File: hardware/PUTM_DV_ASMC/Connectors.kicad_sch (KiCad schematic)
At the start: 7 parts, among them J1 FTSH-107-01-L-D-K, J2 IPBS-110-01-T-D-GP

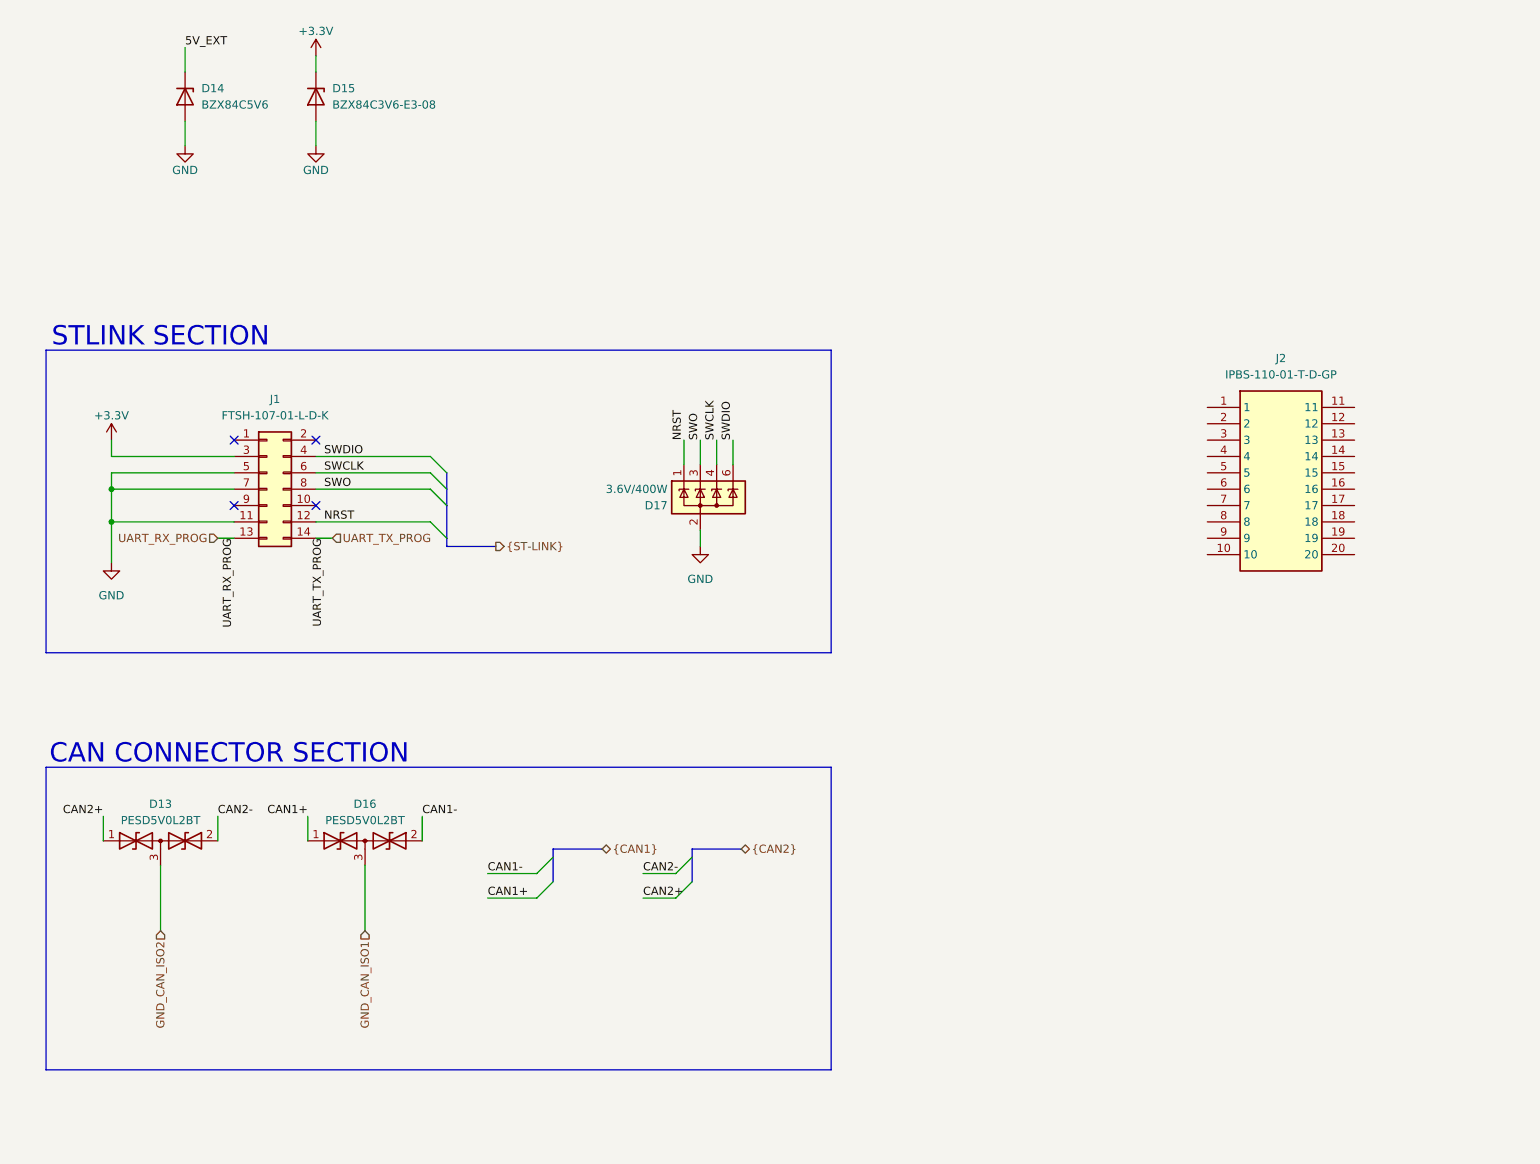
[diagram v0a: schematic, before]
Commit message: done schematic v1
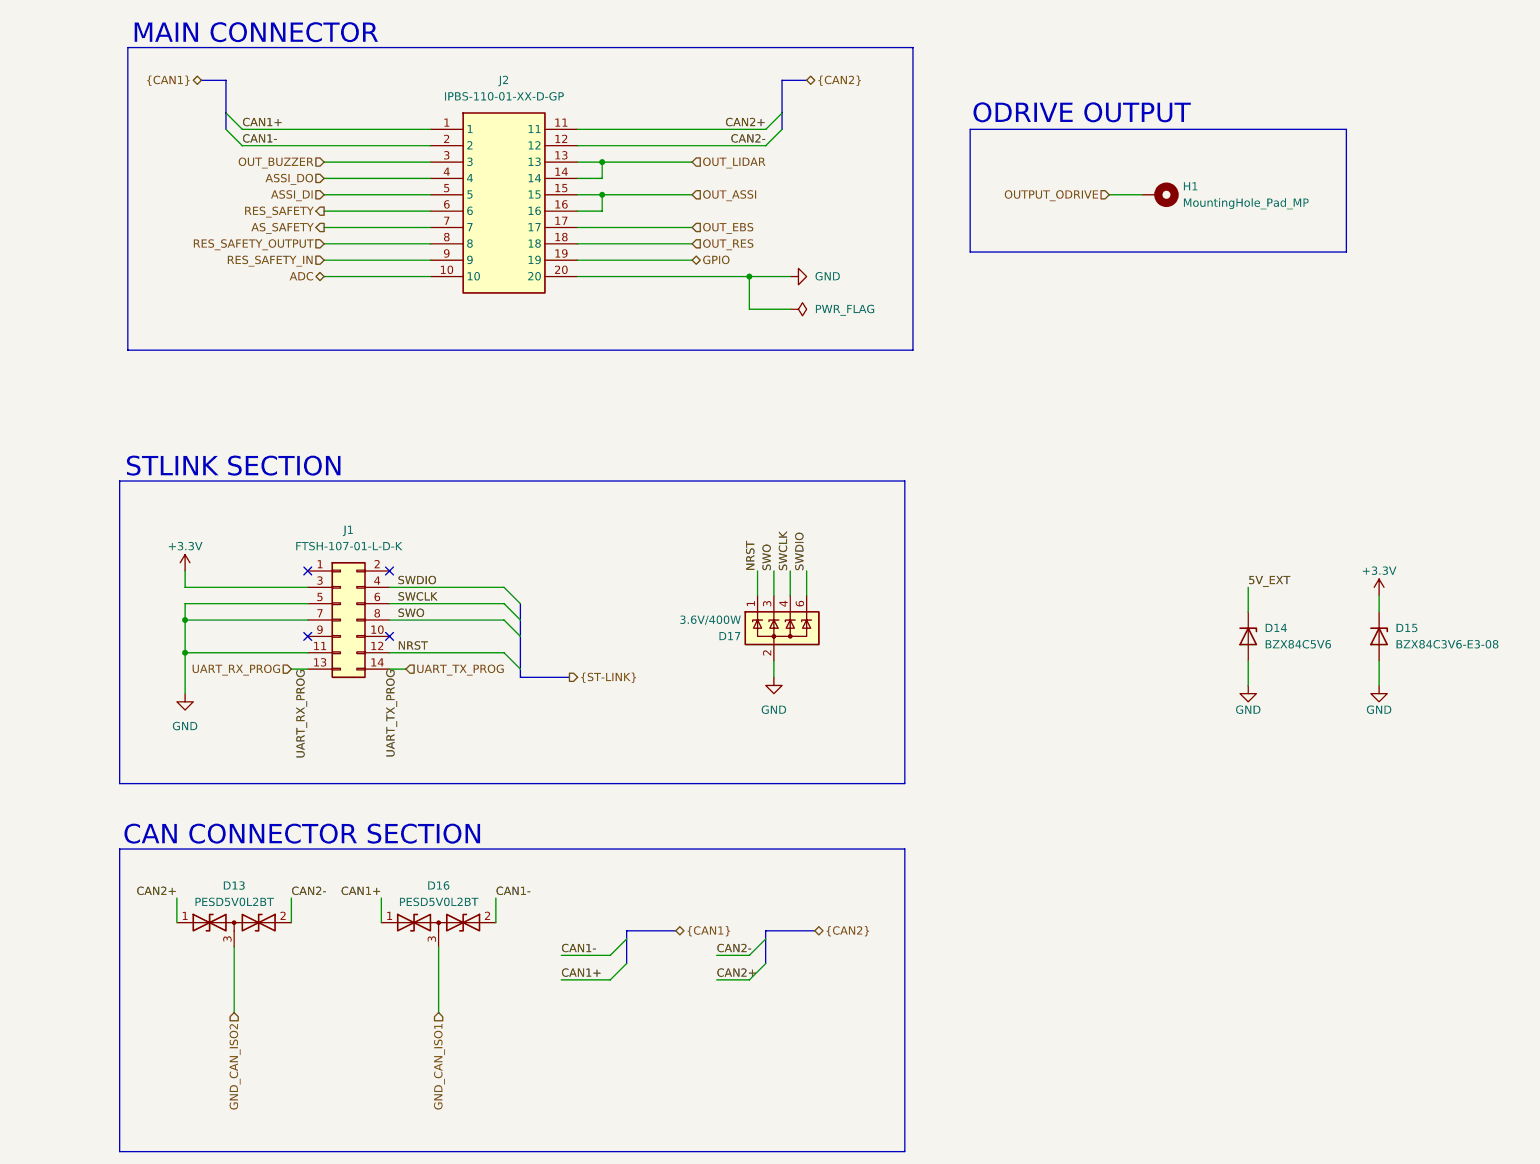
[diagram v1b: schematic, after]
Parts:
- removed J2: IPBS-110-01-T-D-GP, IPBS11001TDGP, symbol IPBS-110-01-T-D-GP:IPBS-110-01-T-D-GP
- added H1: MountingHole_Pad_MP, MountingHole:MountingHole_4.3mm_M4_DIN965_Pad_TopOnly, symbol Mechanical:MountingHole_Pad_MP
- added J2: IPBS-110-01-XX-D-GP, PDM:IPBT110H1TDRAGP, symbol PDM:IPBS-110-01-T-D-GP
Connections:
- net CAN1+: now also J2.1
- net CAN1-: now also J2.2
- net CAN2+: now also J2.11
- net CAN2-: now also J2.12
- net GND: now also J2.20
- new net ADC: J2.10
- new net ASSI_DI: J2.5
- new net ASSI_DO: J2.4
- new net AS_SAFETY: J2.7
- new net GPIO: J2.19
- new net OUTPUT_ODRIVE: H1.MP
- new net OUT_ASSI: J2.15, J2.16
- new net OUT_BUZZER: J2.3
- new net OUT_EBS: J2.17
- new net OUT_LIDAR: J2.13, J2.14
- new net OUT_RES: J2.18
- new net RES_SAFETY: J2.6
- new net RES_SAFETY_IN: J2.9
- new net RES_SAFETY_OUTPUT: J2.8
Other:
- note added: "MAIN CONNECTOR"
- note added: "ODRIVE OUTPUT"
- moved on the sheet: D13, D14, D15, D16, D17, J1
